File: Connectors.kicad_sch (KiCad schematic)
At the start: 5 parts, among them J1 GD820HTX75P6HB, J2 2-338069-0, J3 Conn_02x06_Top_Bottom, J4 Conn_02x06_Top_Bottom, J5 Conn_02x06_Top_Bottom

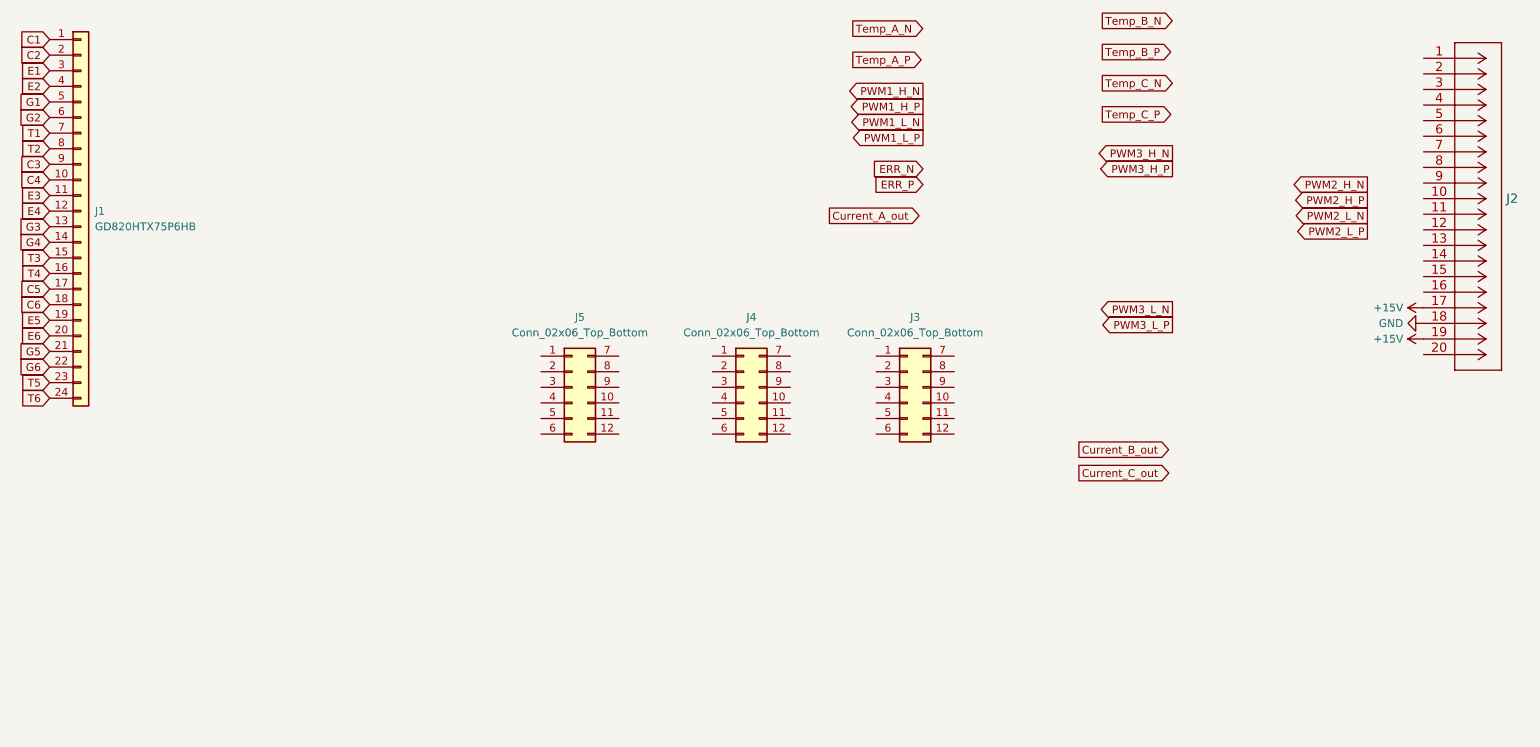
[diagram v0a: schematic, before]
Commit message: Развел вторую стойку
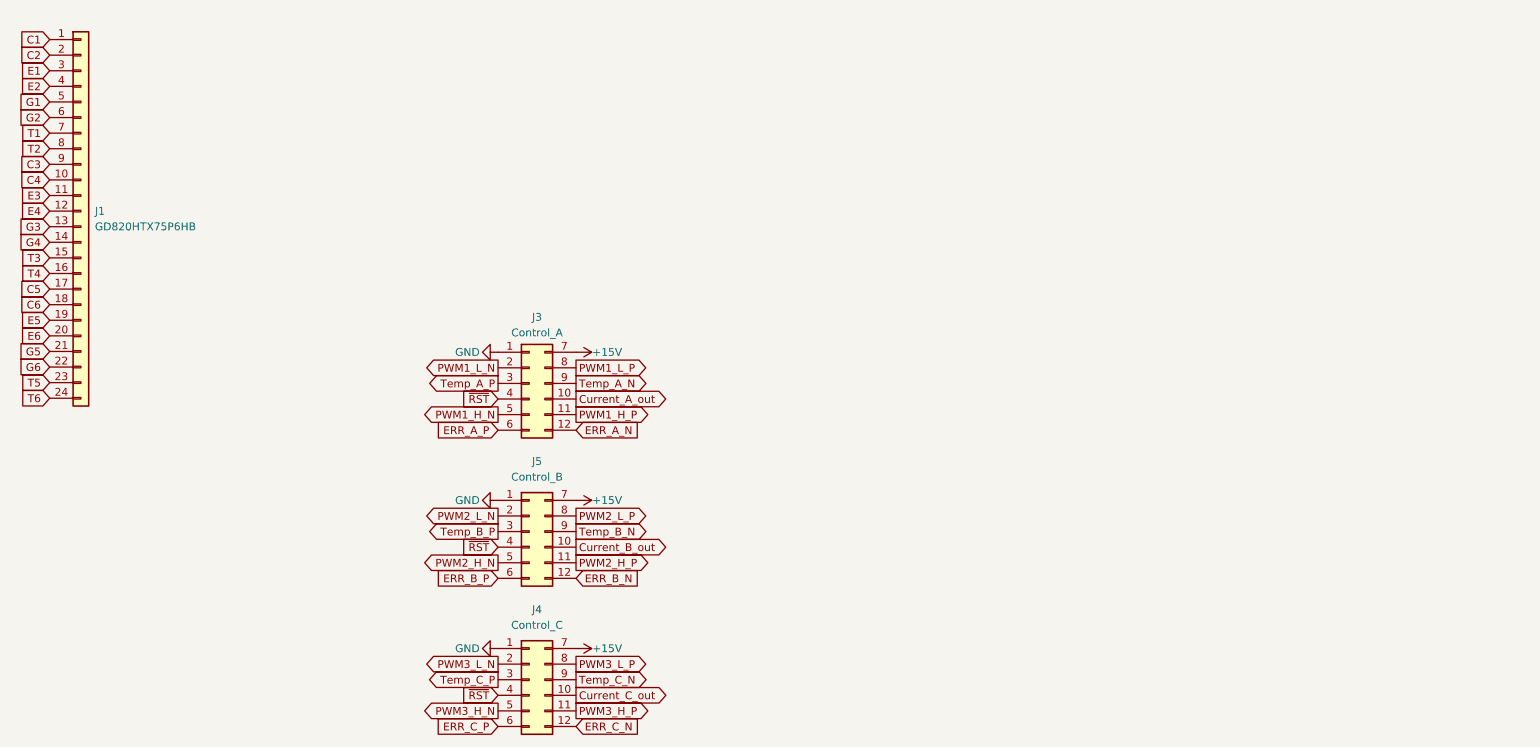
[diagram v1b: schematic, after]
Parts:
- removed J2: 2-338069-0, Connector_My:2-338069-0, symbol Connector_My:2-338069-0
- J3: renamed from J5; value Conn_02x06_Top_Bottom -> Control_A
- J4: renamed from J3; value Conn_02x06_Top_Bottom -> Control_C
- J5: renamed from J4; value Conn_02x06_Top_Bottom -> Control_B
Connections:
- net +15V: now also J3.7 (Pin_7), J4.7 (Pin_7), J5.7 (Pin_7)
- net Current_A_out: now also J3.10 (Pin_10)
- net Current_B_out: now also J5.10 (Pin_10)
- net Current_C_out: now also J4.10 (Pin_10)
- net GND: now also J3.1 (Pin_1), J4.1 (Pin_1), J5.1 (Pin_1)
- net PWM1_H_N: now also J3.5 (Pin_5)
- net PWM1_H_P: now also J3.11 (Pin_11)
- net PWM1_L_N: now also J3.2 (Pin_2)
- net PWM1_L_P: now also J3.8 (Pin_8)
- net PWM2_H_N: now also J5.5 (Pin_5)
- net PWM2_H_P: now also J5.11 (Pin_11)
- net PWM2_L_N: now also J5.2 (Pin_2)
- net PWM2_L_P: now also J5.8 (Pin_8)
- net PWM3_H_N: now also J4.5 (Pin_5)
- net PWM3_H_P: now also J4.11 (Pin_11)
- net PWM3_L_N: now also J4.2 (Pin_2)
- net PWM3_L_P: now also J4.8 (Pin_8)
- net Temp_A_N: now also J3.9 (Pin_9)
- net Temp_A_P: now also J3.3 (Pin_3)
- net Temp_B_N: now also J5.9 (Pin_9)
- net Temp_B_P: now also J5.3 (Pin_3)
- net Temp_C_N: now also J4.9 (Pin_9)
- net Temp_C_P: now also J4.3 (Pin_3)
- net ERR_C_N: now reaches J4.12 (Pin_12)
- net ~{RST}: now reaches J4.4 (Pin_4)
- net ~{RST}: now also J3.4 (Pin_4), J5.4 (Pin_4)
- net ERR_C_P: now reaches J4.6 (Pin_6)
- net ERR_A_N: now reaches J3.12 (Pin_12)
- net ERR_A_P: now reaches J3.6 (Pin_6)
- net ERR_B_N: now reaches J5.12 (Pin_12)
- net ERR_B_P: now reaches J5.6 (Pin_6)
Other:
- moved on the sheet: J3, J4, J5
